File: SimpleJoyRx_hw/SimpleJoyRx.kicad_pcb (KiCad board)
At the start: 2 copper layers, 24 x 60 mm, 111 parts, among them Q1 IRF9358, Q2 2N7002, Q3 IRLML0030, Q4 IRLML0030, SW1 DIPx8, SW2 BUTTON, SW3 1P2T, U1 USBLC6

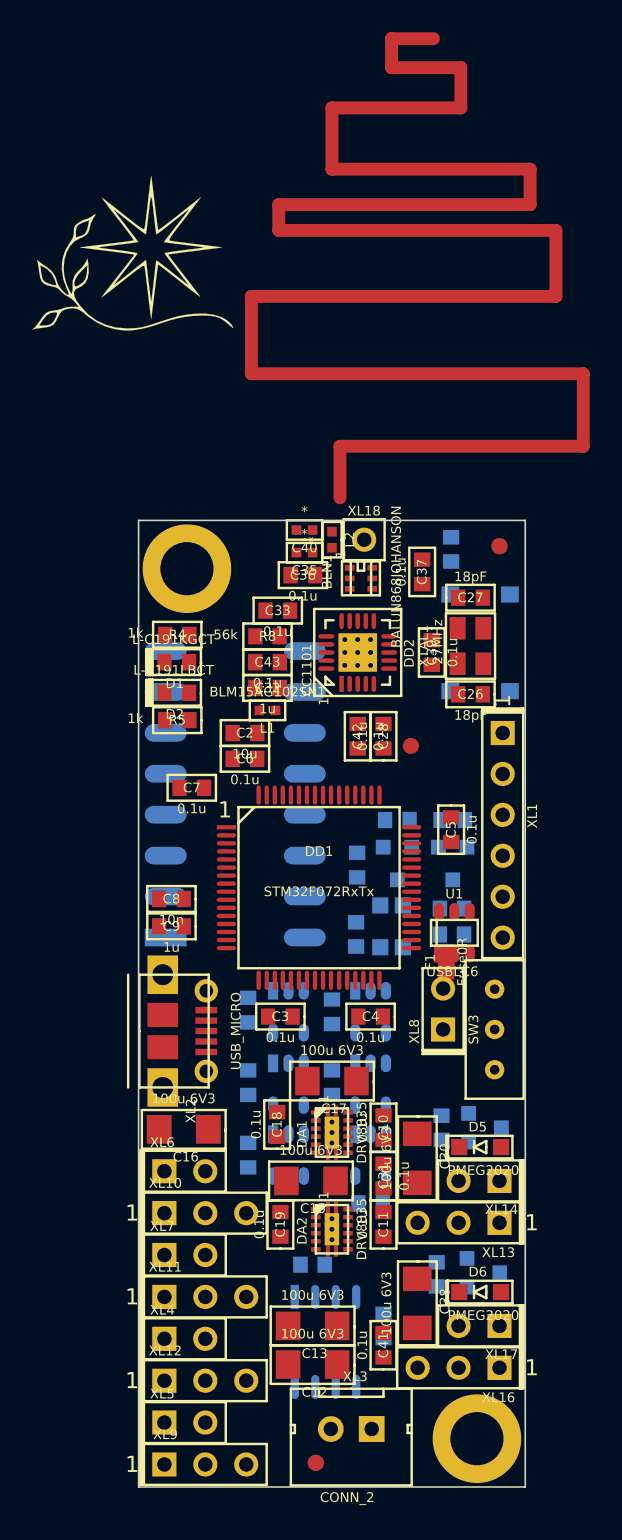
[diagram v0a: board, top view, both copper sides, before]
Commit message: Rx tracing done
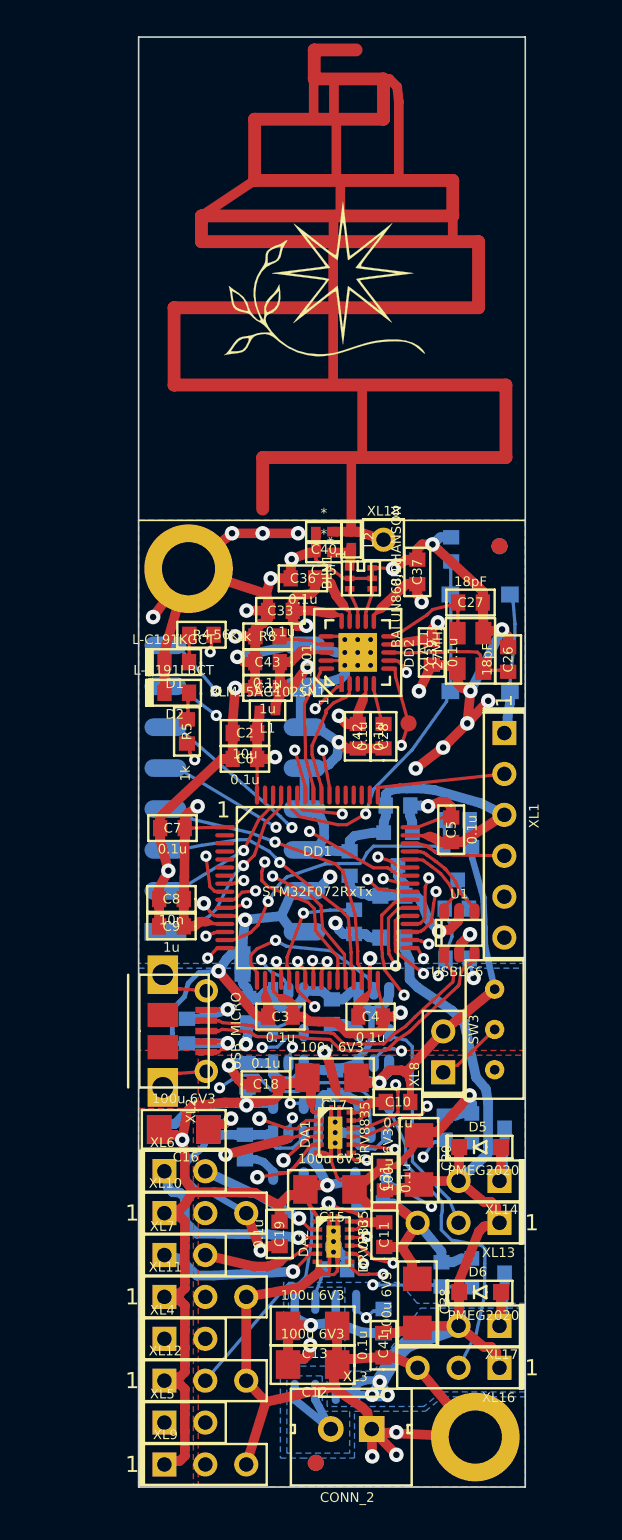
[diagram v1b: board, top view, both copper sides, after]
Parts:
- F1: moved to B.Cu
- moved F1 12.6 mm to (130.5, 97.5)
- moved Logo1 12.0 mm to (135.5, 55.0)
- moved ANT1 4.85 mm to (136.2, 69.7)
- moved C26 3.19 mm to (146.9, 78.6), turned to 90 degrees
- moved C7 2.77 mm to (126.1, 89.1)
- moved XL8 2.66 mm to (142.9, 104.3)
- moved C18 2.60 mm to (131.9, 105.0), turned to 0 degrees
- moved C10 1.84 mm to (140.1, 106.1), turned to 180 degrees
- moved R9 1.54 mm to (143.8, 97.2)
- moved R4 1.50 mm to (127.9, 77.1), turned to 0 degrees
- moved R1 1.42 mm to (136.2, 116.5), turned to 0 degrees
- moved TP1 1.41 mm to (140.8, 82.6)
- moved C15 1.29 mm to (135.9, 111.5)
- moved C40 1.20 mm to (135.5, 70.7)
- moved C35 1.20 mm to (135.5, 72.0)
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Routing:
- net PwrUnst: track 0.00 -> 218.3 mm, vias 0 -> 7
- net GND: track 0.00 -> 212.4 mm, vias 0 -> 28
- net GNDPWR: track 0.00 -> 203.5 mm, vias 0 -> 8
- net /ANT2: track 0.00 -> 147.7 mm
- net +3.3V: track 0.00 -> 119.4 mm, vias 0 -> 6
- net VCC: track 0.00 -> 54.8 mm, vias 0 -> 5
- net +BATT: track 0.00 -> 42.8 mm, vias 0 -> 3
- net /PWM6: track 0.00 -> 28.7 mm, vias 0 -> 2
- net Net-(Q1-Pad4): track 0.00 -> 28.4 mm, vias 0 -> 1
- net /DIR2: track 0.00 -> 28.2 mm, vias 0 -> 2
- net /PWM2: track 0.00 -> 28.1 mm, vias 0 -> 2
- net /PWM1: track 0.00 -> 28.1 mm, vias 0 -> 2
- net /DIR1: track 0.00 -> 27.9 mm, vias 0 -> 2
- net /CC_CS: track 0.00 -> 27.5 mm, vias 0 -> 2
- net /CC_GDO0: track 0.00 -> 27.4 mm, vias 0 -> 2
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- added copper zone on B.Cu, net +BATT
- added copper zone on B.Cu, net /PRE_BAT_PWR
- added copper zone on B.Cu, net GND
- added copper zone on F.Cu, net GND
- added copper zone on In1.Cu, net GND
- added copper zone on In2.Cu, net GND
- added copper zone on B.Cu, net GNDPWR
- added copper zone on F.Cu, net GNDPWR
- added copper zone on In1.Cu, net GNDPWR
- added copper zone on In2.Cu, net GNDPWR
- added copper zone on B.Cu, net PwrUnst
- added copper zone on F.Cu, net PwrUnst
- added copper zone on In1.Cu, net PwrUnst
- added copper zone on In2.Cu, net PwrUnst
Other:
- board size 24 x 60 mm -> 24 x 90 mm
- copper layers 2 -> 4
- net class Default: clearance 0.2 -> 0.21; trace_width 0.2 -> 0.25; via_dia 0.8 -> 0.7; via_drill 0.4 -> 0.3
- net class Wide added: clearance 0.21, trace_width 0.6, via_dia 0.9, via_drill 0.4
- rule trace_clearance: 0.2 -> 0.21
- rule trace_min: 0.2 -> 0.1
- rule via_min_drill: 0.3 -> 0.2
- rule via_min_size: 0.4 -> 0.3
